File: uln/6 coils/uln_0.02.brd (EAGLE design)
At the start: 44.1 x 41.9 mm, 8 parts, among them IC1 ULN2003AD, IC2 74HC595D, IC3 ULN2003AD, J1 4P-2.0, J2 4P-2.0, J3 4P-2.0

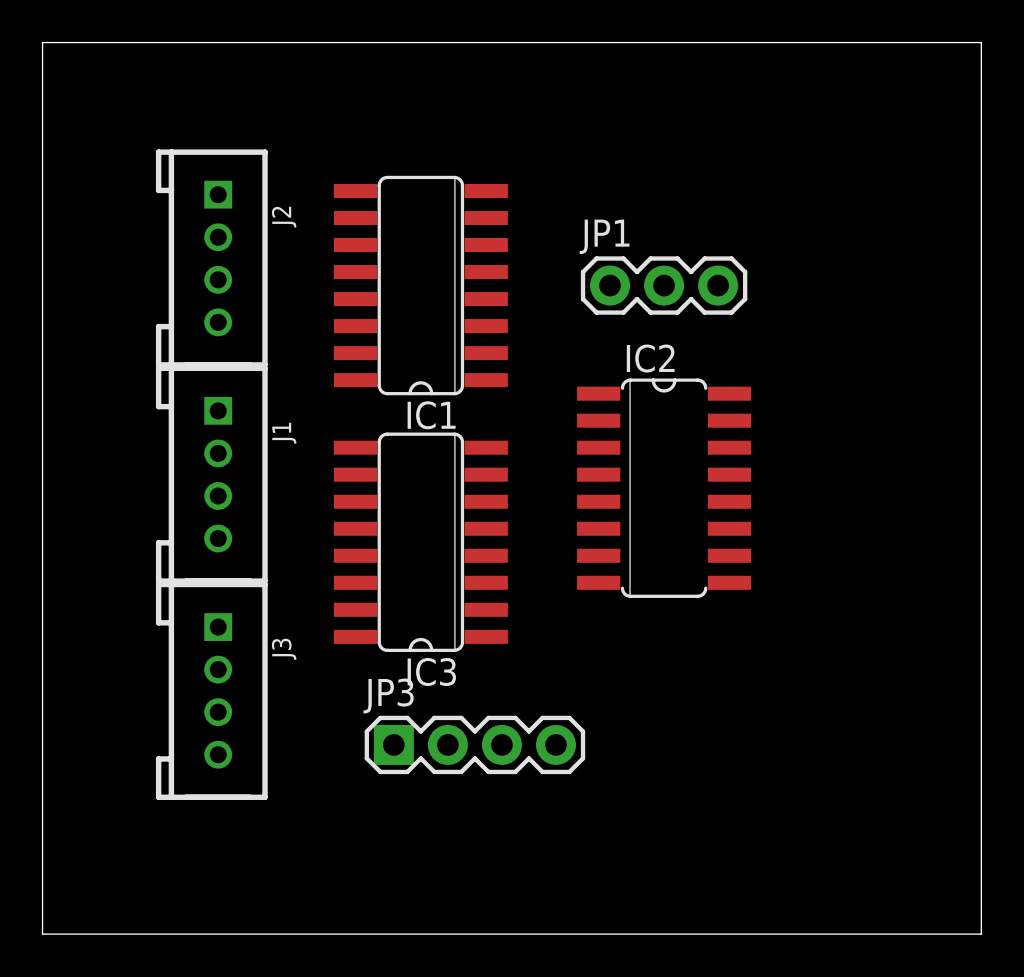
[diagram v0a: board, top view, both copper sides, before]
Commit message: Updated uln2003 and l298 board
Last version ;)
Ready to be made at the hva lab
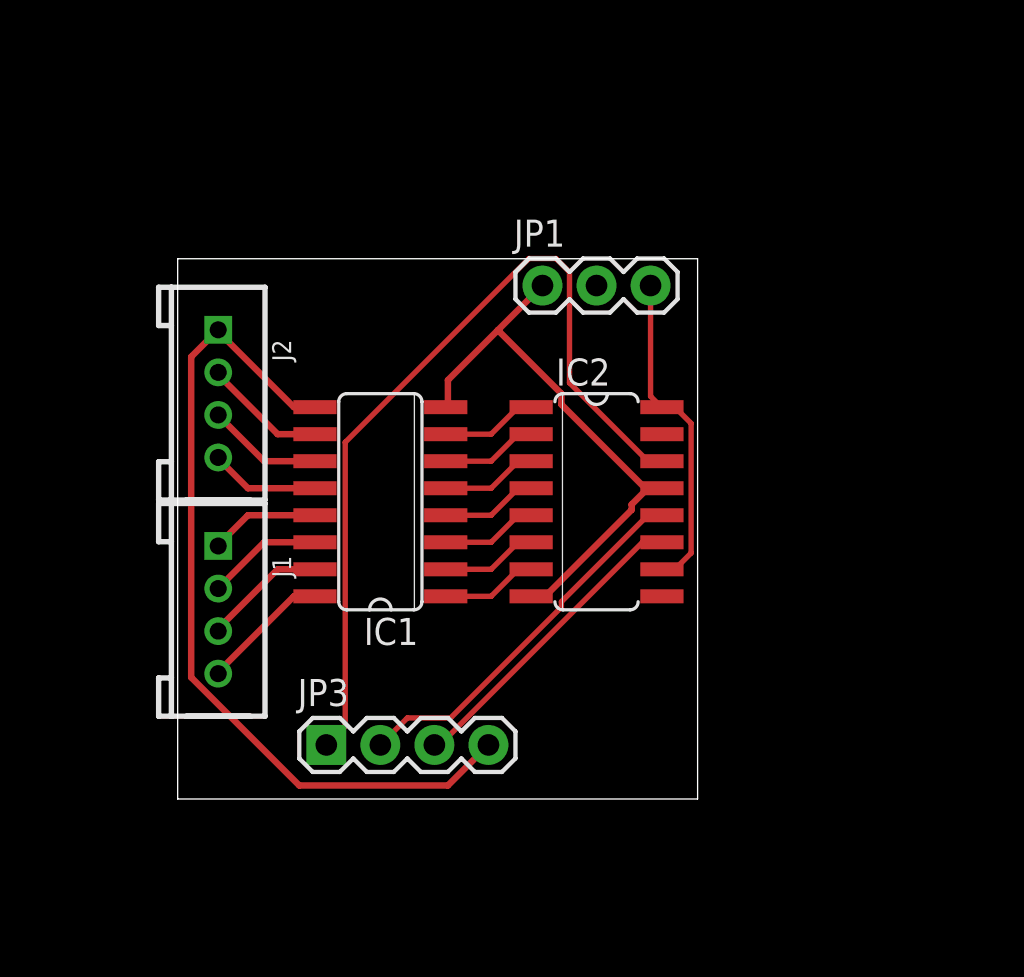
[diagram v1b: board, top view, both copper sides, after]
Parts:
- removed IC3: ULN2003AD, uln-udn:SO16
- removed J3: 4P-2.0, Seeed-OPL-Connector:HW4-2.0
- moved IC1 10.3 mm to (9.53, 14.0)
- moved J1 6.35 mm to (1.91, 8.89)
- moved J2 6.35 mm to (1.91, 19.1)
- moved IC2 3.24 mm to (19.7, 14.0)
- moved JP1 3.18 mm to (17.1, 24.1)
- moved JP3 3.17 mm to (6.99, 2.54)
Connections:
- removed net N$16: IC3.14, J3.1
- removed net N$8: IC2.15, IC3.3
- net GND: no longer IC3.8
- net VCC: no longer IC3.9
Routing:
- net N$19: track 0.00 -> 40.0 mm
- net VCC: track 0.00 -> 39.9 mm
- net GND: track 0.00 -> 27.1 mm
- net N$18: track 0.00 -> 17.9 mm
- net 5V: track 0.00 -> 15.4 mm
- net N$17: track 0.00 -> 14.6 mm
- net N$15: track 0.00 -> 6.10 mm
- net N$9: track 0.00 -> 5.81 mm
- net N$14: track 0.00 -> 5.81 mm
- net N$10: track 0.00 -> 5.46 mm
- net N$13: track 0.00 -> 5.46 mm
- net N$12: track 0.00 -> 5.17 mm
- net N$11: track 0.00 -> 5.17 mm
- net N$5: track 0.00 -> 4.54 mm
- net N$7: track 0.00 -> 4.54 mm
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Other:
- board size 44.1 x 41.9 mm -> 24.4 x 25.4 mm
